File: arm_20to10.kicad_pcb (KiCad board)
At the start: 2 copper layers, 29 x 30 mm, 12 parts, among them J1 Conn_ARM_JTAG_SWD_20, J2 Conn_ARM_JTAG_SWD_10, SW1 SW_SPDT, SW2 SW_SPST, U1 TLV70033_SOT23-5

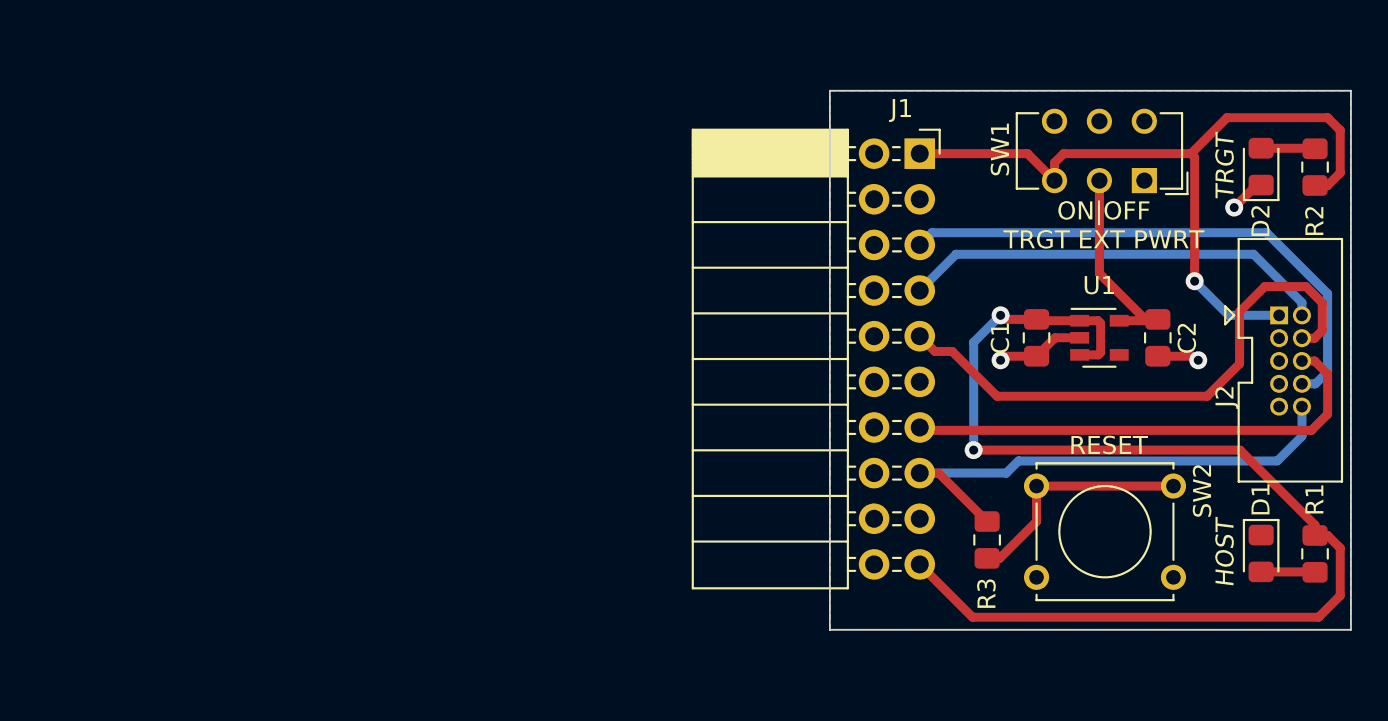
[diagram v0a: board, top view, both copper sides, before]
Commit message: Progressed PCB layout.
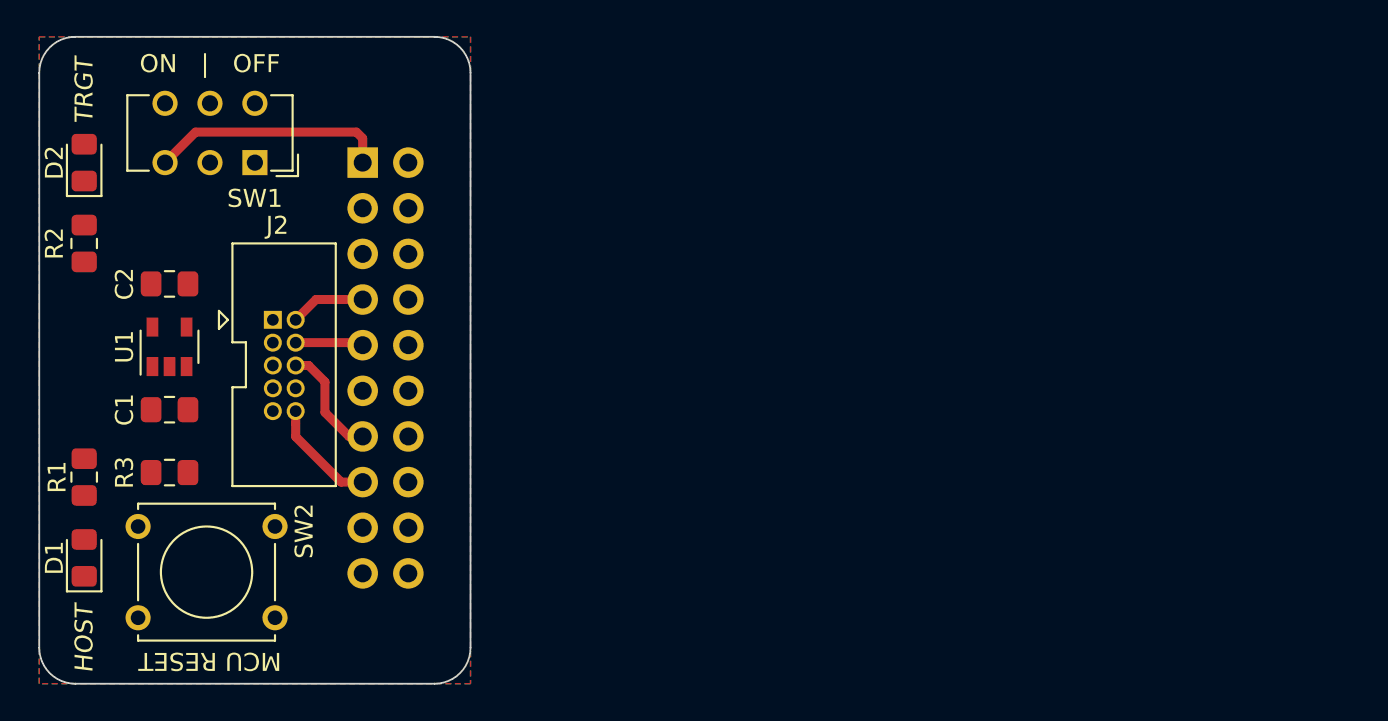
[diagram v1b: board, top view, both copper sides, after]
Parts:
- J1: footprint Connector_PinSocket_2.54mm:PinSocket_2x10_P2.54mm_Horizontal -> Connector_PinSocket_2.54mm:PinSocket_2x10_P2.54mm_Vertical; moved to B.Cu
- moved R1 68.6 mm to (119.5, 146.5)
- moved R2 68.6 mm to (119.5, 133.5)
- moved D1 65.5 mm to (119.5, 151.0), turned to 90 degrees
- moved D2 65.5 mm to (119.5, 129.0)
- moved J2 56.0 mm to (130.0, 137.8)
- moved C2 55.1 mm to (124.2, 135.8), turned to 0 degrees
- moved U1 51.8 mm to (124.2, 139.2), turned to 90 degrees
- moved SW2 50.1 mm to (122.5, 149.2)
- moved SW1 49.5 mm to (129.0, 129.0)
- moved C1 48.4 mm to (124.2, 142.8), turned to 180 degrees
- moved R3 45.7 mm to (124.2, 146.2), turned to 180 degrees
- moved J1 31.0 mm to (135.0, 129.0), turned to 180 degrees
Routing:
- net /5V: track 67.5 -> 0.00 mm, vias 2 -> 0
- net /TDI: track 30.4 -> 0.00 mm
- net /VCC: track 43.1 -> 13.2 mm, vias 1 -> 0
- net /SWCLK: track 31.2 -> 3.79 mm
- net /~RESET: track 28.6 -> 6.20 mm
- net /SWO: track 27.1 -> 6.36 mm
- net /SWDIO: track 23.9 -> 4.20 mm
- net Net-(R3-Pad2): track 13.2 -> 0.00 mm
- net Net-(C2-Pad1): track 11.7 -> 0.00 mm
- net /GND: track 9.28 -> 0.00 mm, vias 3 -> 0
- net Net-(D2-Pad2): track 3.01 -> 0.00 mm
- net Net-(D1-Pad2): track 3.01 -> 0.00 mm
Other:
- board size 29 x 30 mm -> 24 x 36 mm
- board text added: "MCU RESET"
- board text added: "ON | OFF"
- board text removed: "ON|OFF TRGT EXT PWRT"
- board text removed: "RESET"
- board text removed: "SWDIO SWCLK SWO NC nRESET"
- board text removed: "VCC GND GND NC GND"
